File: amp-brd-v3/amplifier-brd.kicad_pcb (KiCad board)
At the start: 4 copper layers, 32.5 x 30 mm, 30 parts, among them J1 VOUT, J2 VOUT, Q1 BSS84, U2 INA233, U3 DS28EA00, U4 LMR36510ADDA

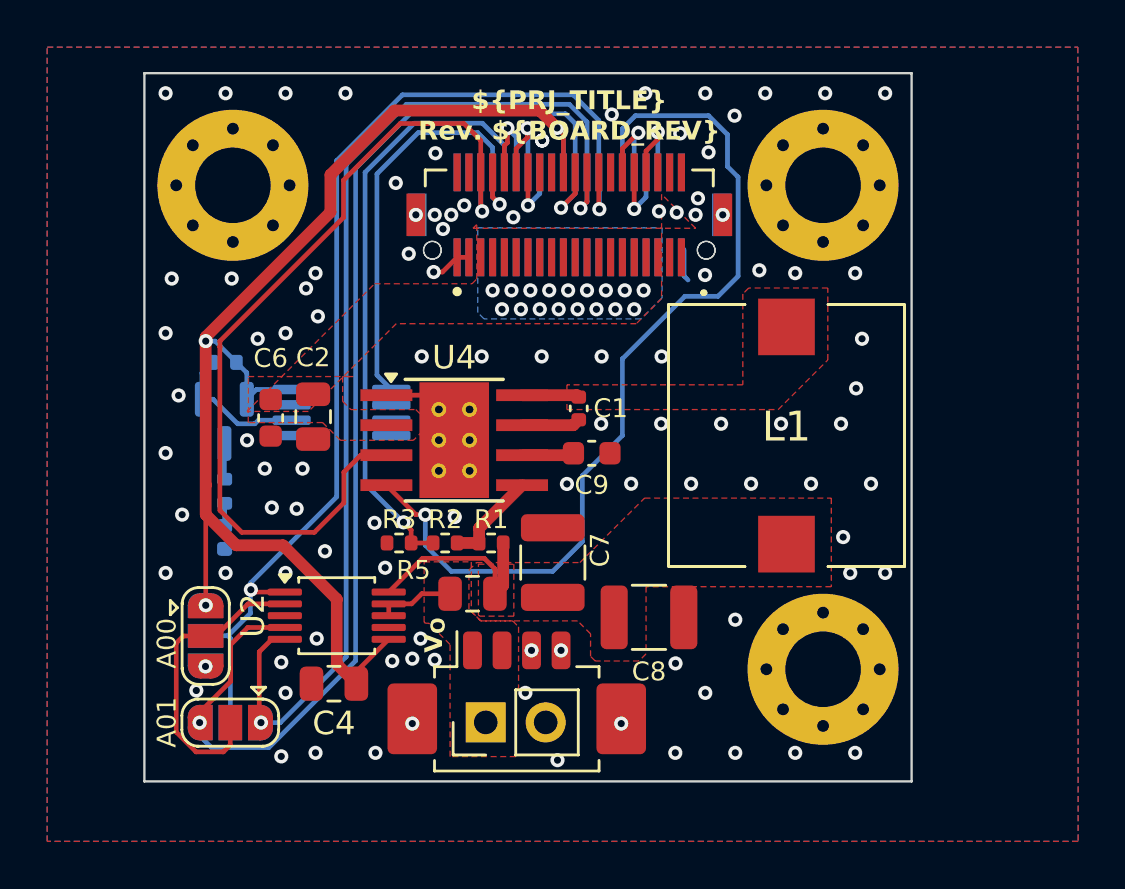
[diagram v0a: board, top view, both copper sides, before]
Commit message: Final review with Joe
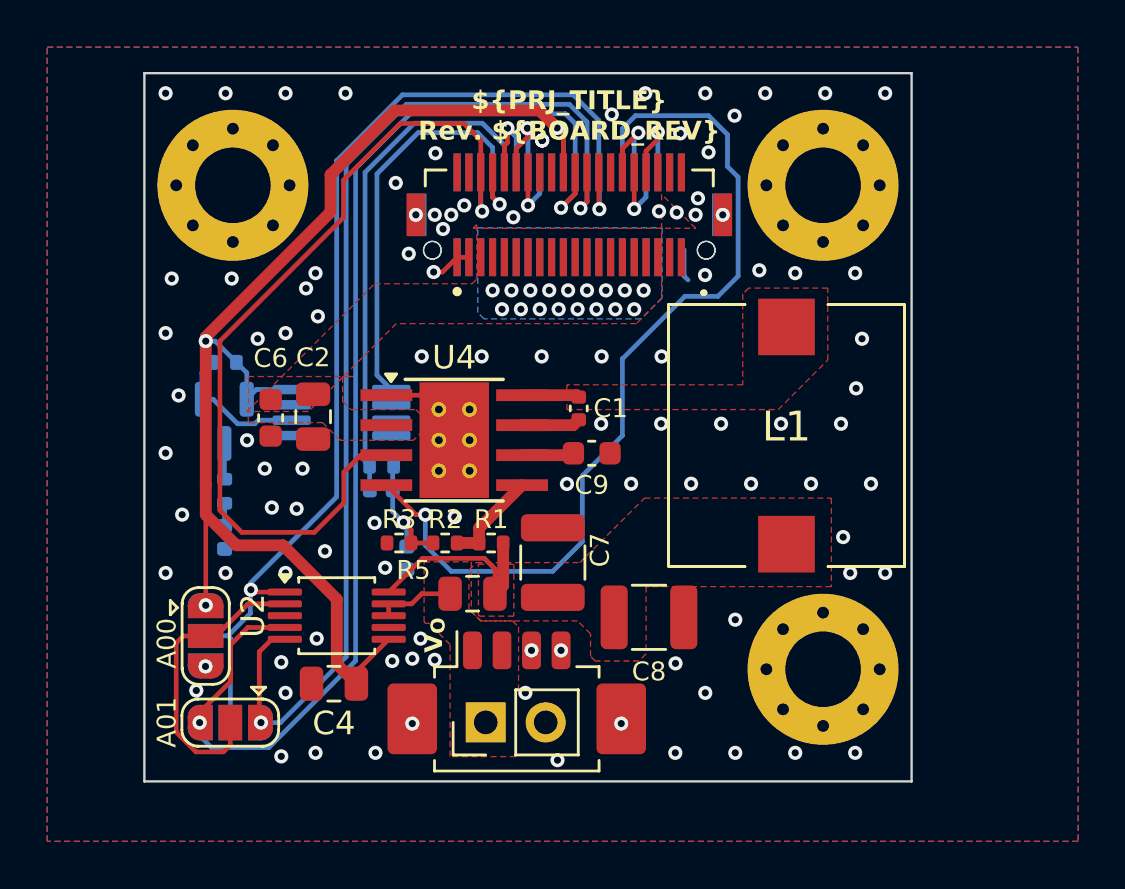
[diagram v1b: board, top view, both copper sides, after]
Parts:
- added D2: D_Schottky, Diode_SMD:D_0402_1005Metric, B.Cu at (224.0, 104.6)
- added D3: D_Schottky, Diode_SMD:D_0402_1005Metric, B.Cu at (222.9, 101.7)
- added R4: 0, Resistor_SMD:R_0402_1005Metric, B.Cu at (222.9, 100.7)
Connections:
- R2 pad 2: /CTRL_A -> /OP AMP/FCTRL
- R3 pad 2: /CTRL_A -> /OP AMP/FCTRL
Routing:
- net /OP AMP/FCTRL: track 0.00 -> 5.61 mm, vias 0 -> 1
- net /CTRL_A: track 25.7 -> 22.1 mm, vias 1 -> 0
